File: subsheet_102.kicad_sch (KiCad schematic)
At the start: 14 parts, among them J7 MIDI IN, J8 MIDI OUT, U35 74LS04_PHY, U39 PC900_PHY

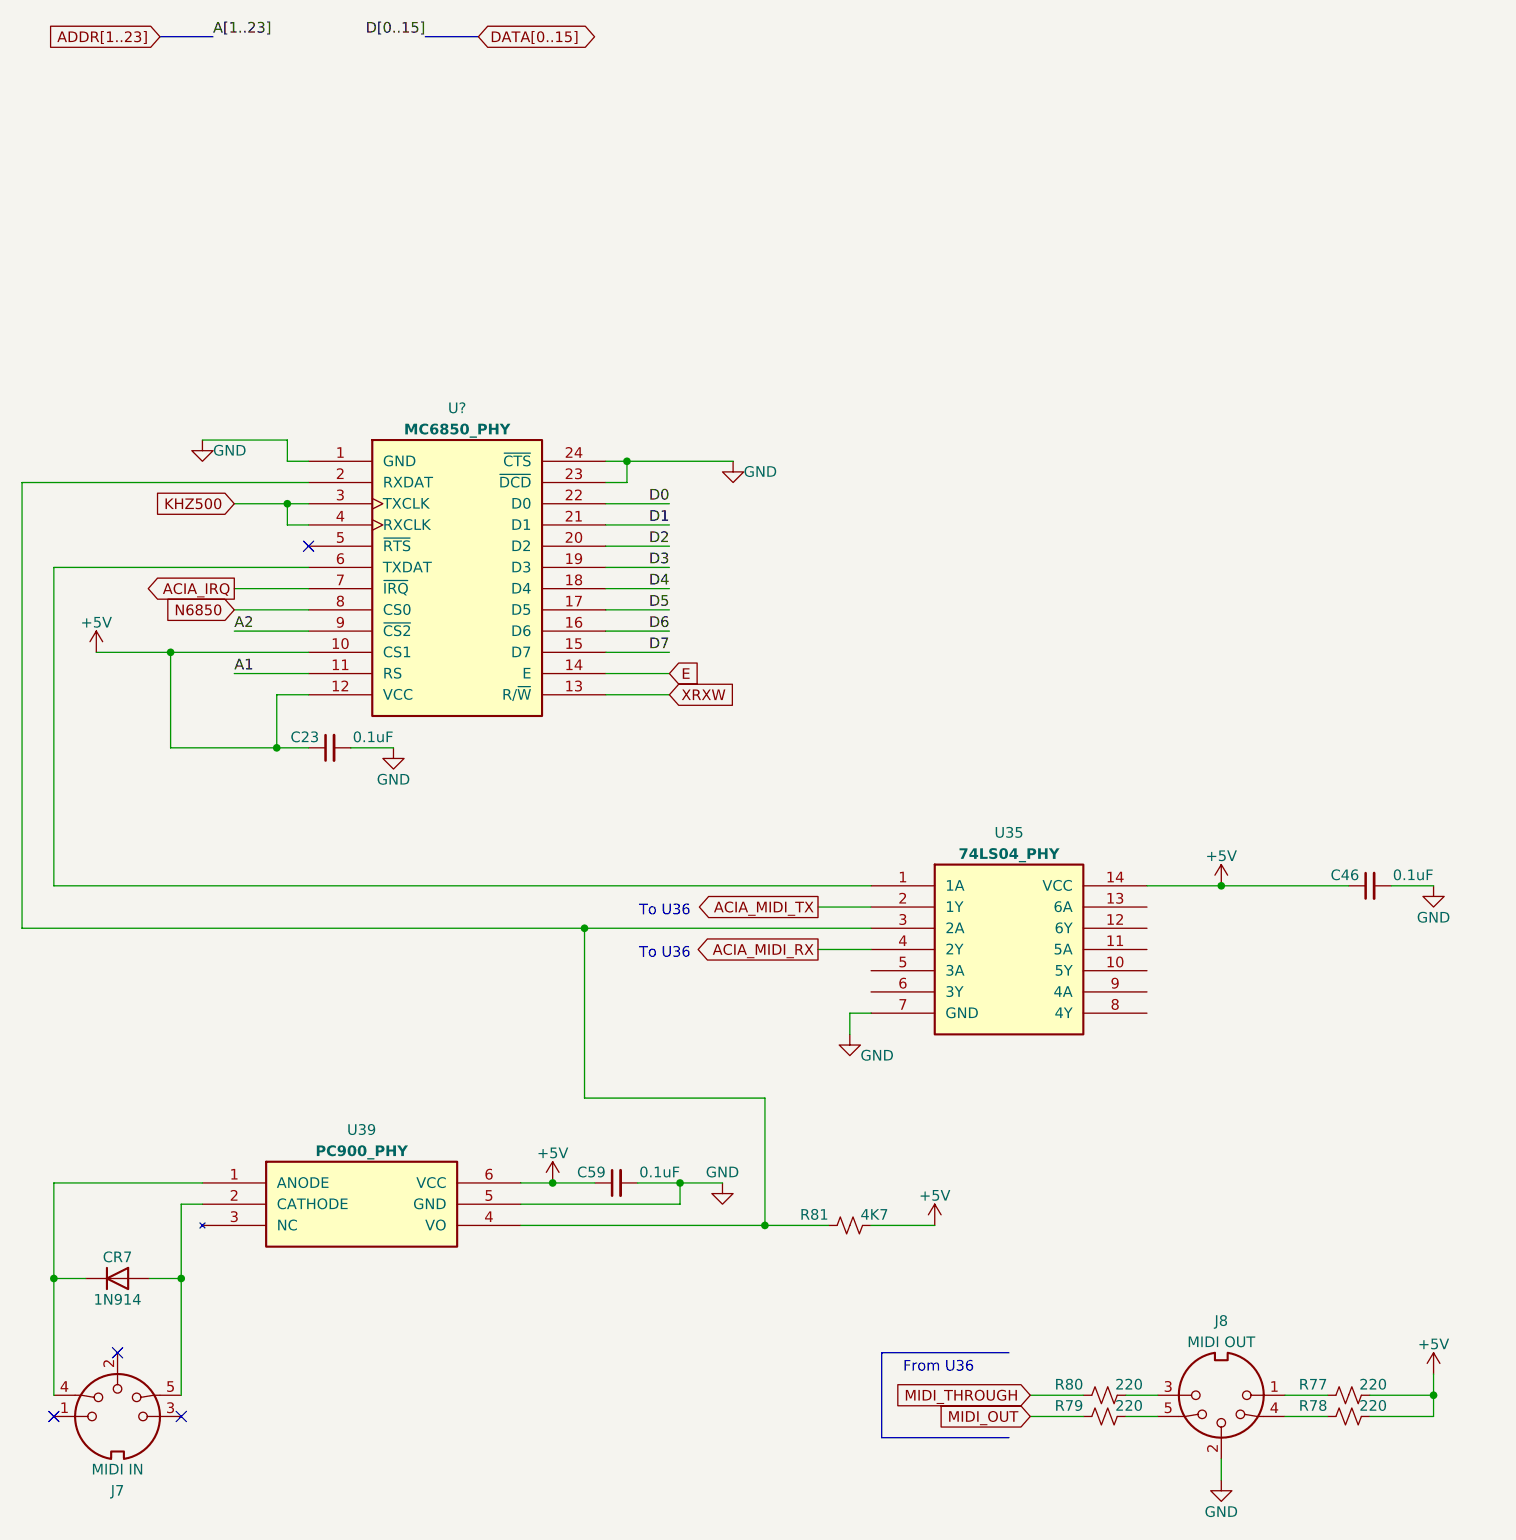
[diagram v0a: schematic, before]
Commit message: done remaining u36
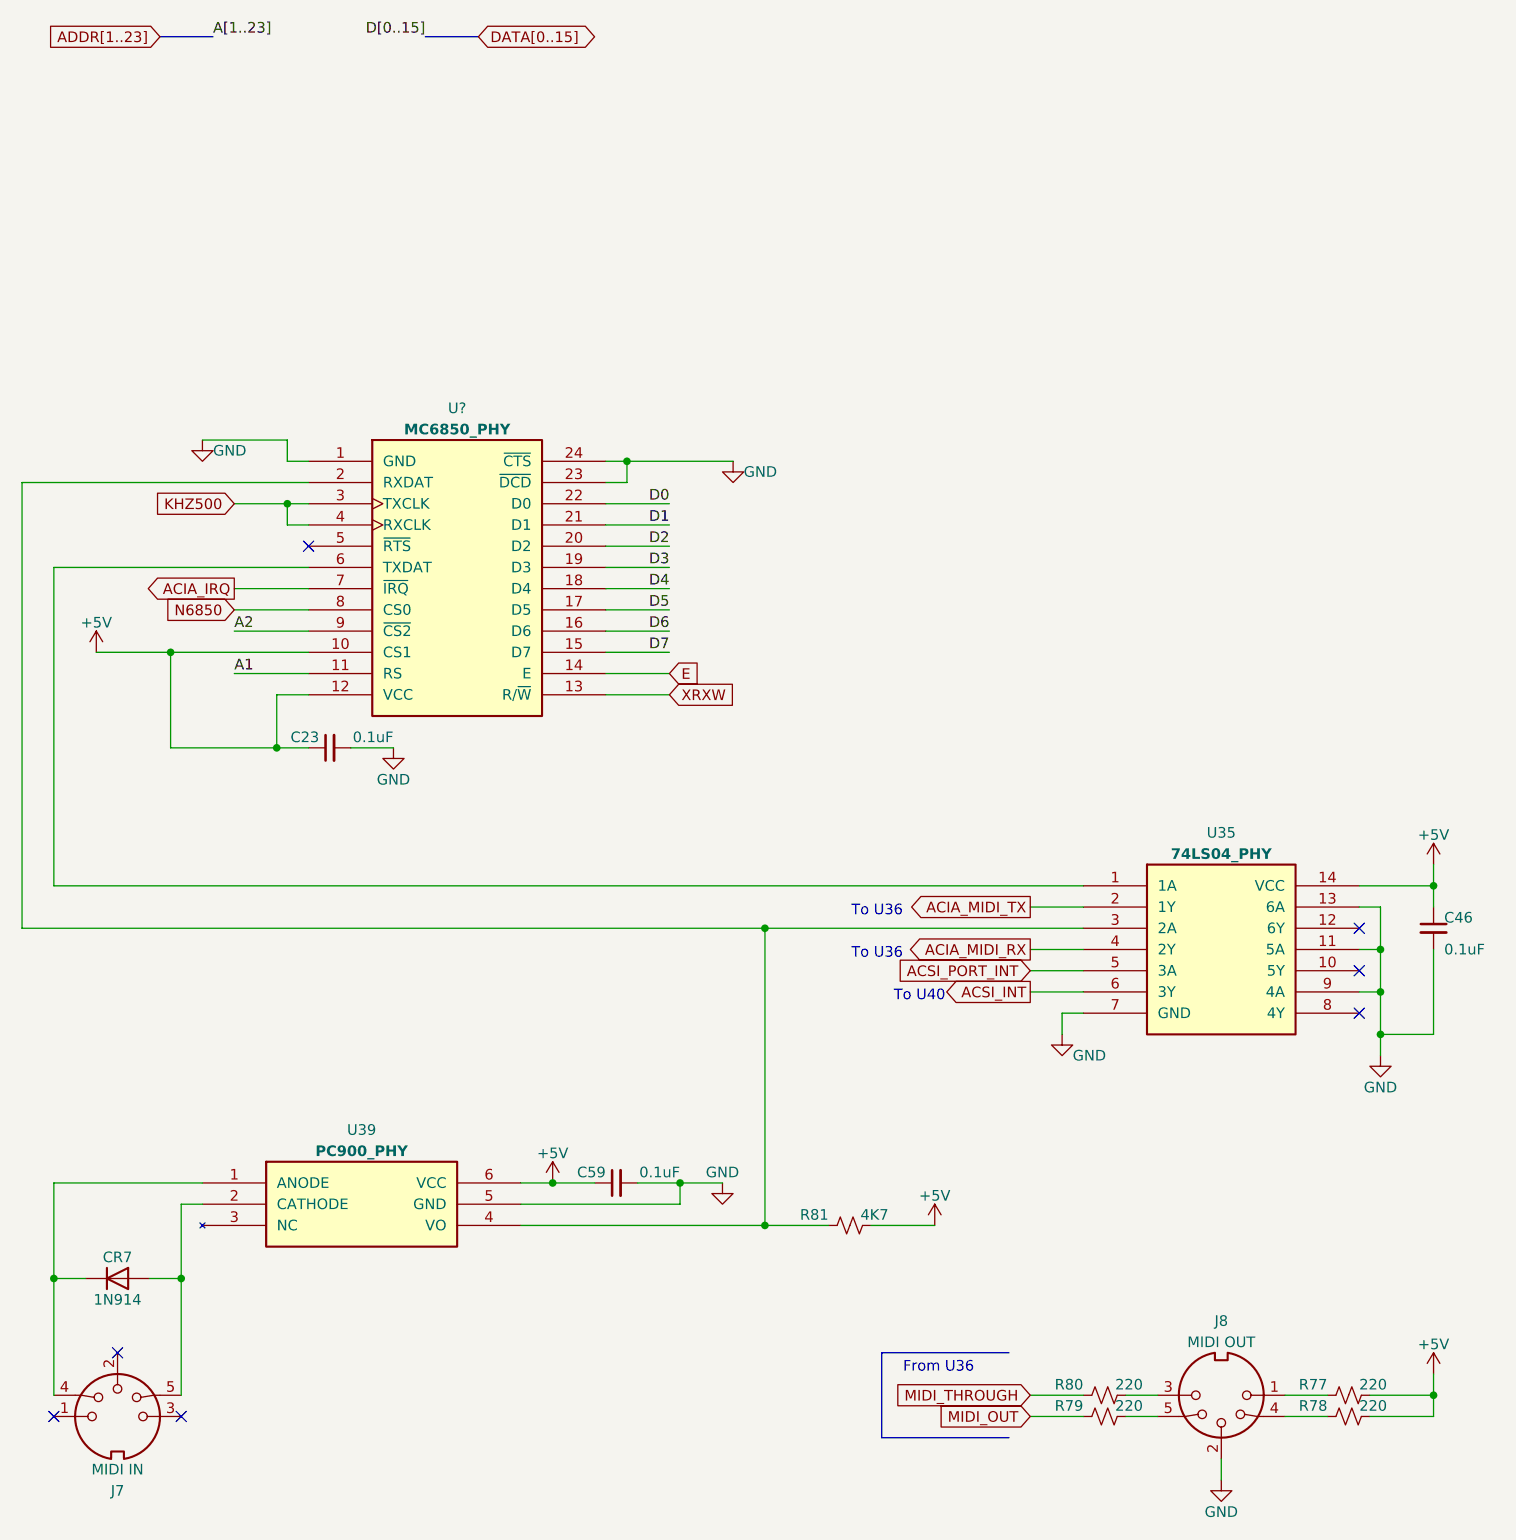
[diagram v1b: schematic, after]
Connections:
- net GND: now also U35.11 (5A), U35.13 (6A), U35.9 (4A)
- net ACSI_PORT_INT: now reaches U35.5 (3A)
- net ACSI_INT: now reaches U35.6 (3Y)
- no-connect marks 4 -> 7
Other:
- note added: "To U40"
- moved on the sheet: C46, U35
